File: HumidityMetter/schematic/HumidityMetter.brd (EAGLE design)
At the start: 100 x 68 mm, 66 parts, among them IC1 LM317, IC2 LM317, IC3 STM32F103C8T6, IC4 AM2320, J1 0, J2 0, J3 0, J4 0, K1 POWER_ON, T1 BSS84, T2 BC847, X1 +9V, X2 GND, X3 ISP

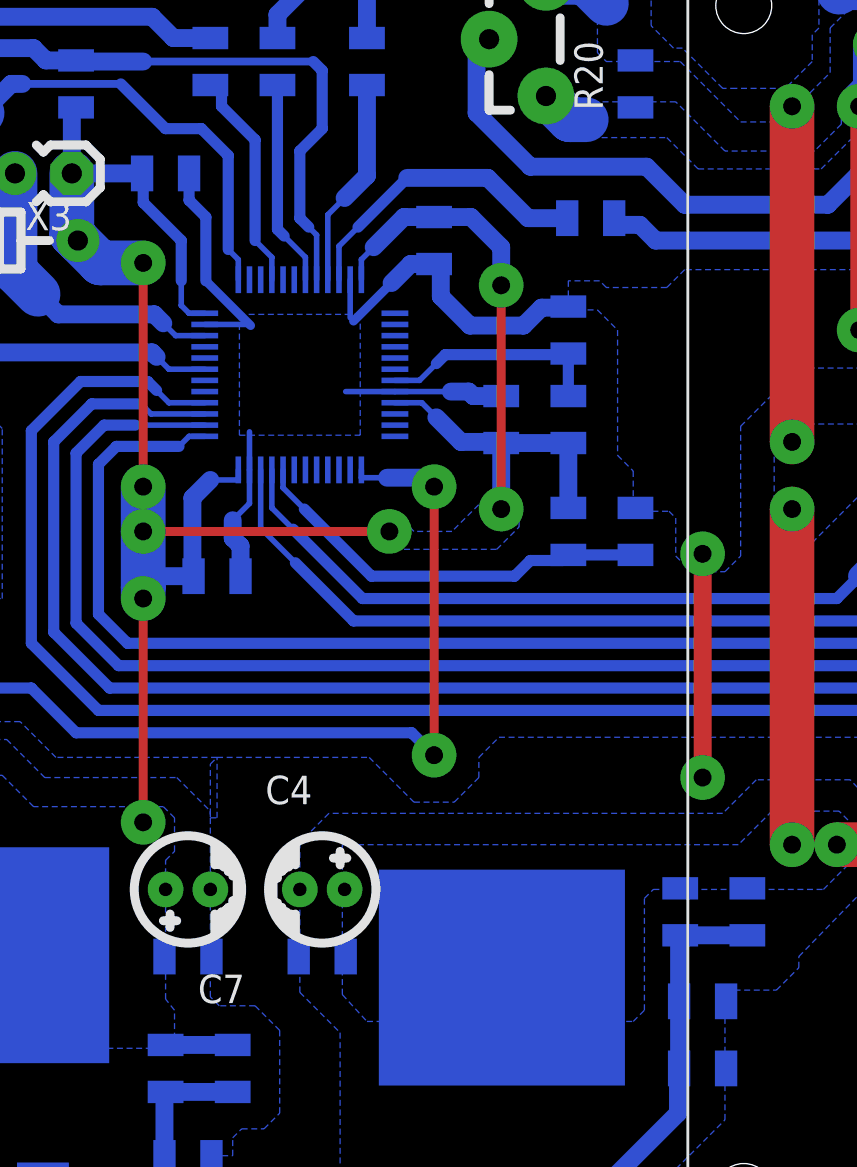
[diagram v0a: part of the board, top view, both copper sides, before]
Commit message: Himidity metter. Board routed. Fix tiny problems.
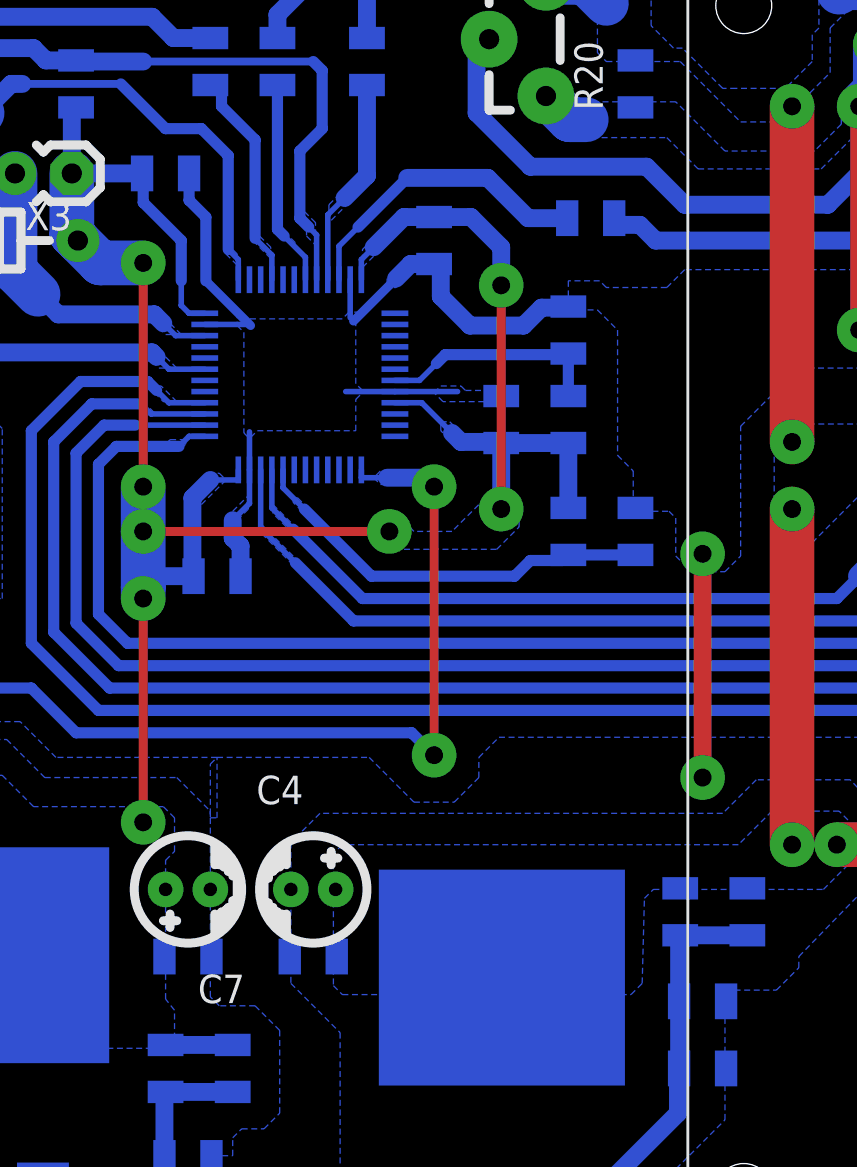
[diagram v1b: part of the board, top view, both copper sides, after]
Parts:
- moved C4 0.40 mm to (36.6, 16.0)
- moved C5 0.40 mm to (36.6, 13.0)
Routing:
- net GND: track 82.4 -> 80.4 mm
- added copper zone on layer 16, net ADC_9V
- added copper zone on layer 16, net BOOT0
- added copper zone on layer 16, net BOOT1
- added copper zone on layer 16, net ERROR_LED
- added copper zone on layer 16, net I2C_SCL
- added copper zone on layer 16, net I2C_SDA
- added copper zone on layer 16, net LCD_D4
- added copper zone on layer 16, net LCD_D5
- added copper zone on layer 16, net LCD_D7
- added copper zone on layer 16, net LCD_E
- added copper zone on layer 16, net LCD_RS
- added copper zone on layer 16, net PWR_HOLD
- added copper zone on layer 16, net SWDCLK
- added copper zone on layer 16, net SWDIO

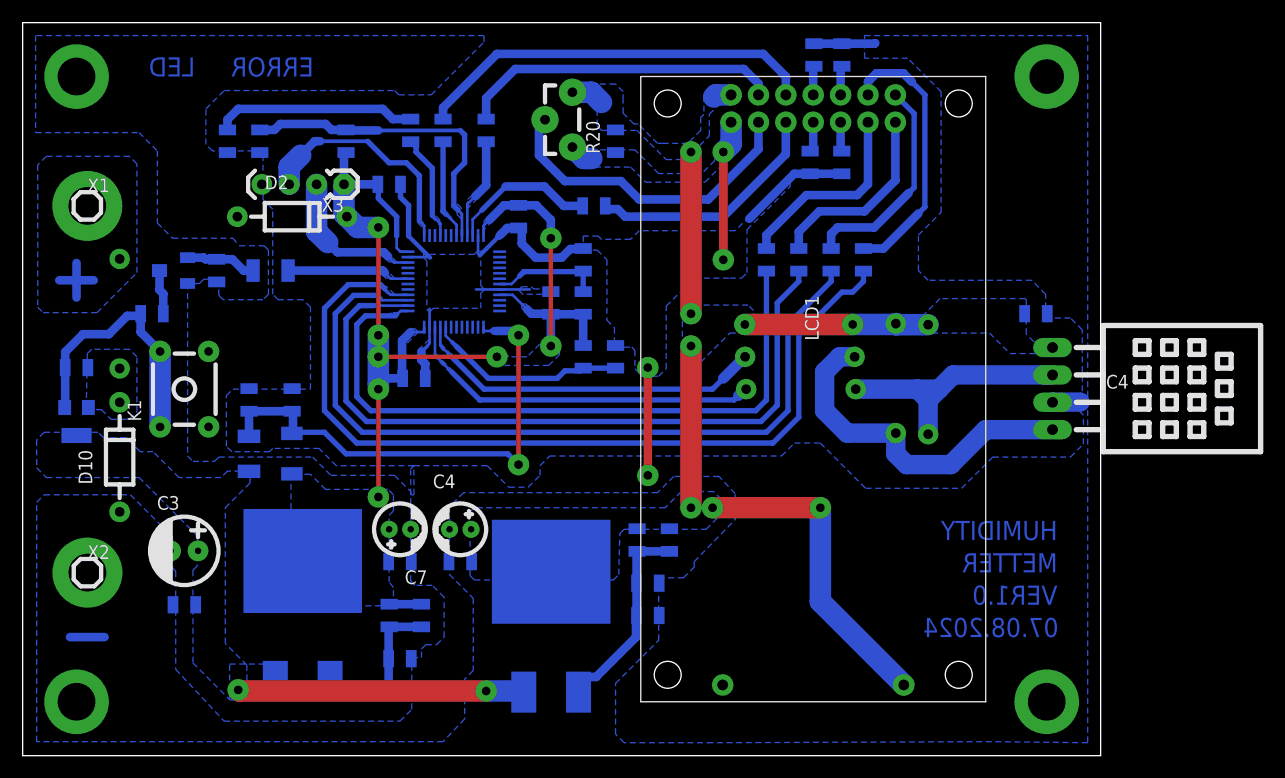
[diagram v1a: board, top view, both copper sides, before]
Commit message: Himidity metter. Board routed. Fix tiny problems.
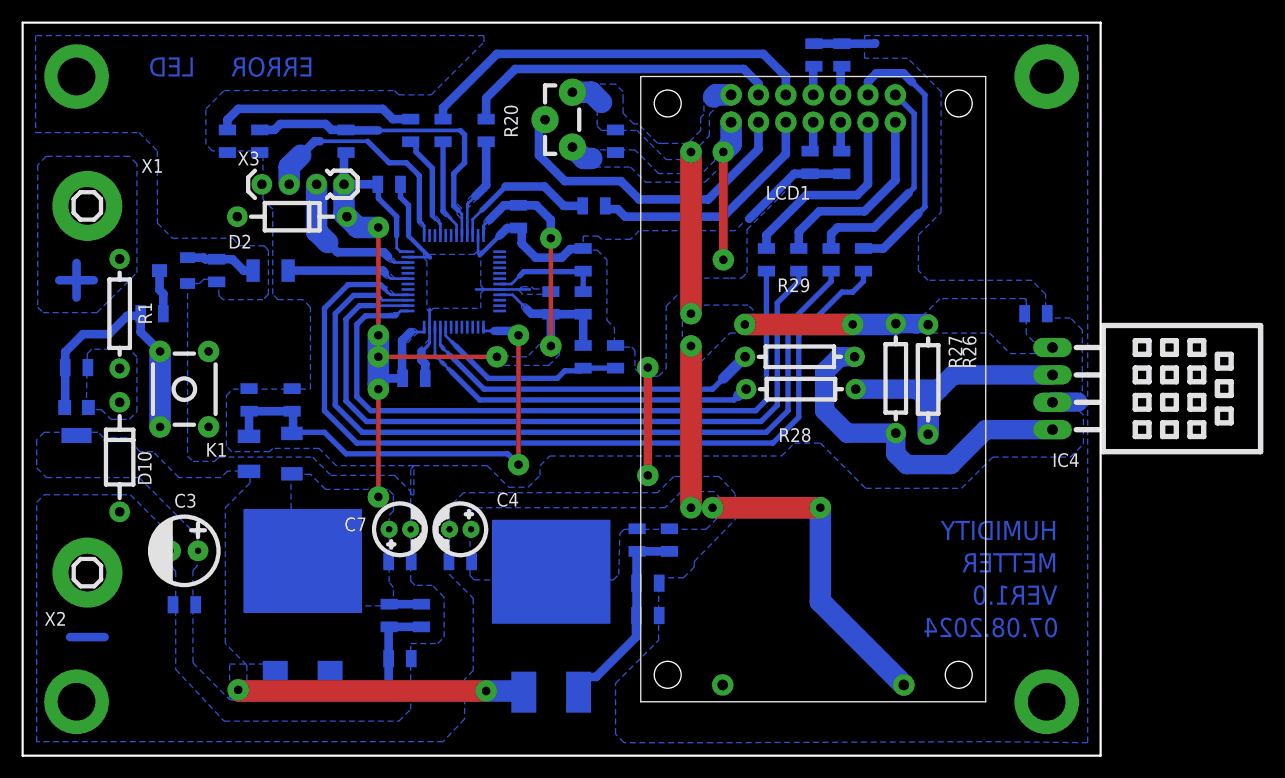
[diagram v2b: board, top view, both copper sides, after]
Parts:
- flipped R1 to the top
- flipped R26 to the top
- flipped R27 to the top
- flipped R28 to the top, turned to 0 degrees
- flipped R29 to the top, turned to 0 degrees
